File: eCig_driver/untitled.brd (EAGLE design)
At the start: 9.4 x 19.5 mm, 5 parts

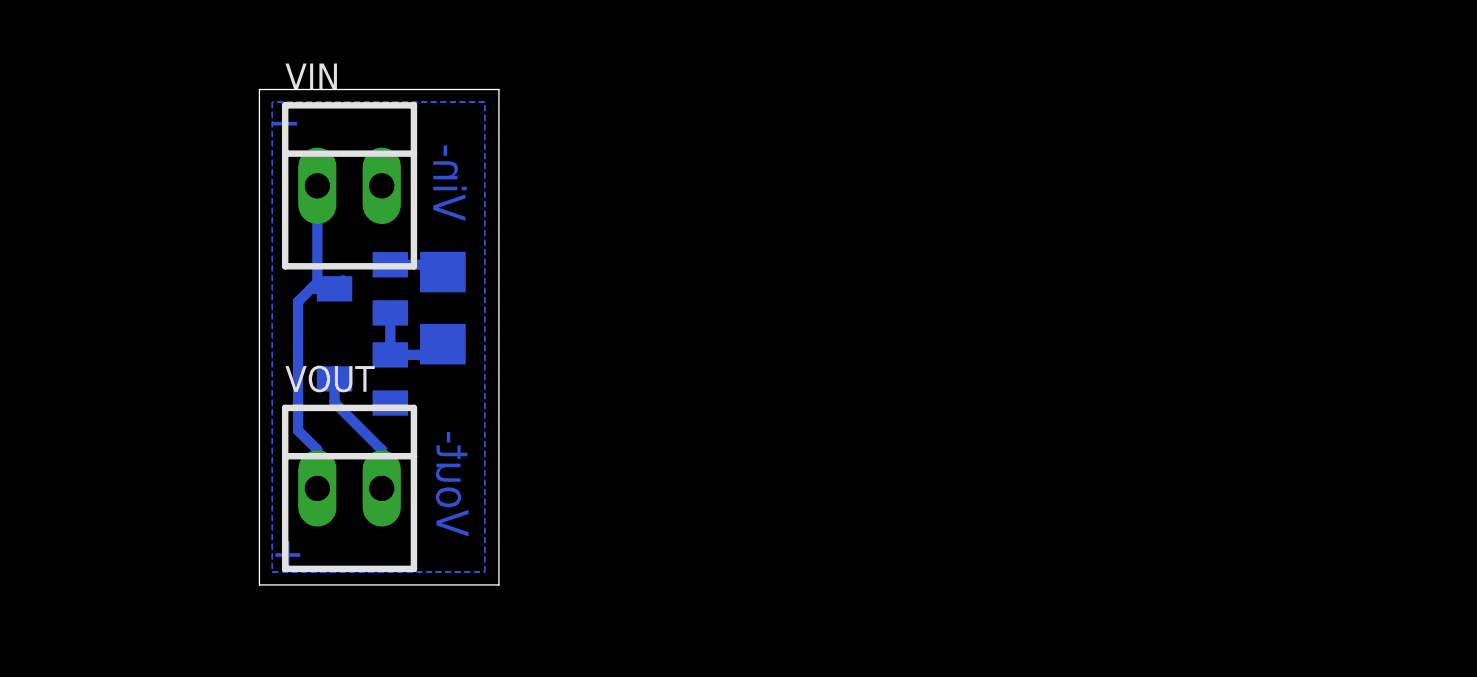
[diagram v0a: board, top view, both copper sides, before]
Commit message: new update podlewacz v2
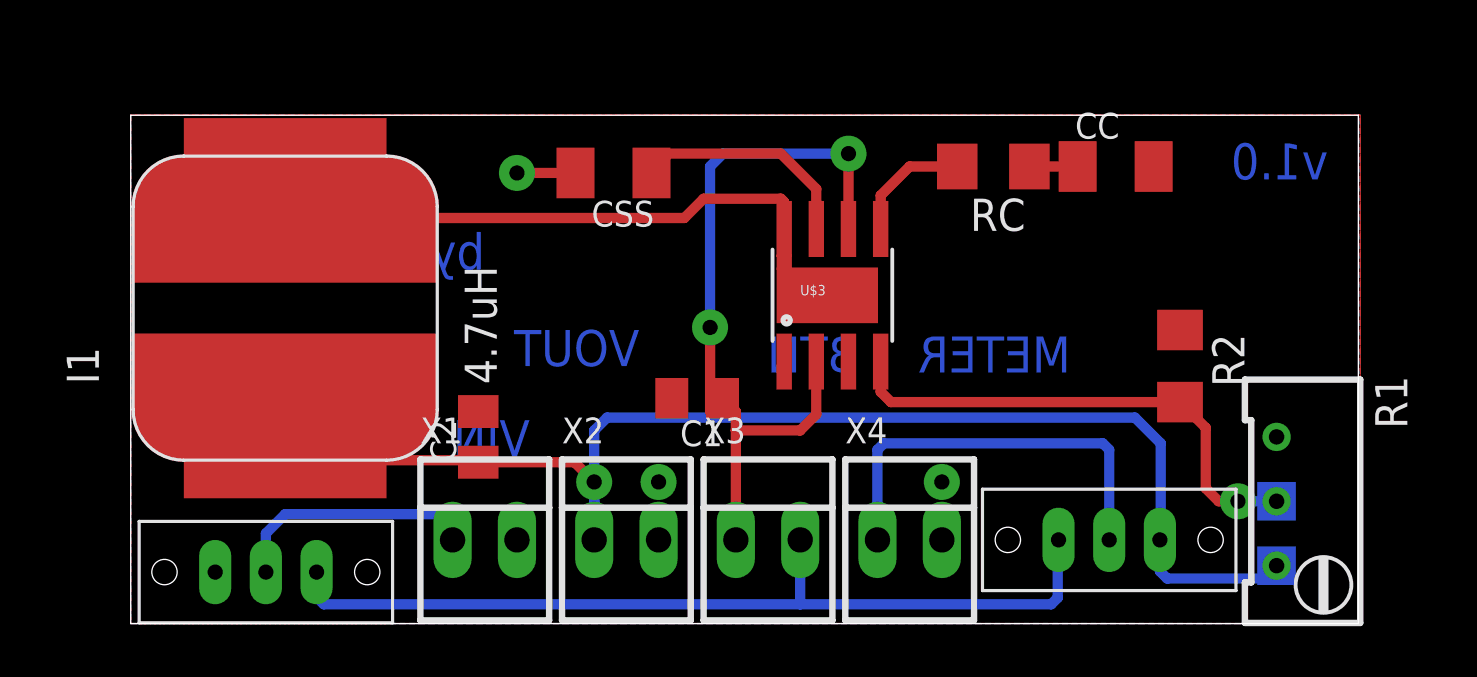
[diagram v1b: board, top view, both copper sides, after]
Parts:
- removed MOSFET: AO3400A, smd-footprints:SOT-23
- removed RESET_IC: (no value), telcom:SOT23B-3
- removed VIN, VOUT: (no value), con-molex:22-23-2021
- added C1: 10uF, resistor:C0805K
- added C2: 22uf, resistor:C0805K
- added CC: 1nf, resistor:C1206K
- added CSS: 10nf, resistor:C1206K
- added I1: 4.7uH, sh4dov lib:RH127
- added MASTER_ON, METER_SWITCH: SPDT_SLIDE_SWITCH_2_PITCH, sh4dov lib:SPDT_SLIDE_SWITCH_2_PITCH
- added R2: 10K, resistor:R1206
- added RC: 22k, resistor:R1206
- added U$3: AOZ1051PI, sh4dov lib:AOZ1051PI
- added X1: VIN, con-molex:22-23-2021
- added X2: VOUT, con-molex:22-23-2021
- added X3: button, con-molex:22-23-2021
- added X4: voltmeter, con-molex:22-23-2021
- R1: value 1k -> 100k; device resistor:R1206 -> resistor:RTRIM64W
- moved R1 35.0 mm to (46.5, 4.83), flipped to the top, turned to 180 degrees
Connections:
- new net N$10: MASTER_ON.S1, METER_SWITCH.S0, X3.2
- new net N$2: CC.1, RC.1
- new net N$4: CSS.1, U$3.7
- new net N$5: METER_SWITCH.COMMON, X4.1
- new net N$6: I1.P$1, U$3.8, U$3.P$1, U$3.P$2
- new net N$7: C2.1, I1.P$2, METER_SWITCH.S1, R1.3, X2.1
- new net N$8: MASTER_ON.COMMON, X1.1
- net GND: now also C1.2, C2.2, CC.2, CSS.2, R2.1, U$3.1, U$3.3, X1.2, X2.2, X4.2; no longer MOSFET.2, R1.2, RESET_IC.1, VIN.2
- net N$1: now also RC.2, U$3.5; no longer MOSFET.3, VOUT.2
- net N$3: now also R1.2, R2.2, U$3.4; no longer MOSFET.1, R1.1, RESET_IC.2
- net VCC: now also C1.1, U$3.2, U$3.6, X3.1; no longer RESET_IC.3, VIN.1, VOUT.1
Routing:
- net N$7: track 0.00 -> 52.1 mm, vias 0 -> 1
- net N$10: track 0.00 -> 35.3 mm
- net N$6: track 0.00 -> 22.1 mm
- net N$5: track 0.00 -> 16.5 mm
- net VCC: track 14.0 -> 30.4 mm, vias 0 -> 2
- net N$3: track 3.91 -> 20.0 mm, vias 0 -> 1
- net N$8: track 0.00 -> 9.92 mm
- net N$4: track 0.00 -> 9.10 mm
- net N$2: track 0.00 -> 1.90 mm
- net GND: track 2.20 -> 2.67 mm, vias 0 -> 3
- added copper zone on layer 1, net GND
- added copper zone on layer 1, net N$11
- added copper zone on layer 16, net N$9
- removed copper zone on layer 16, net N$2
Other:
- board size 9.4 x 19.5 mm -> 48.4 x 20.1 mm
- board text added: "BTN"
- board text added: "METER"
- board text added: "VIN"
- board text added: "VOUT"
- board text added: "by Sh4DoV"
- board text added: "master"
- board text added: "v1.0"
- board text removed: "+"
- board text removed: "Vin-"
- board text removed: "Vout-"
